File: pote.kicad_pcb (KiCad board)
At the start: 2 copper layers, 39.4 x 36.8 mm, 16 parts, among them J1 Conn_01x01, J2 Conn_01x01, J3 Conn_01x01, J4 Conn_01x01, J5 Conn_01x01, J6 Conn_01x01, J7 Conn_01x01, J8 Conn_01x01, U1 Opamp_Quad_Generic

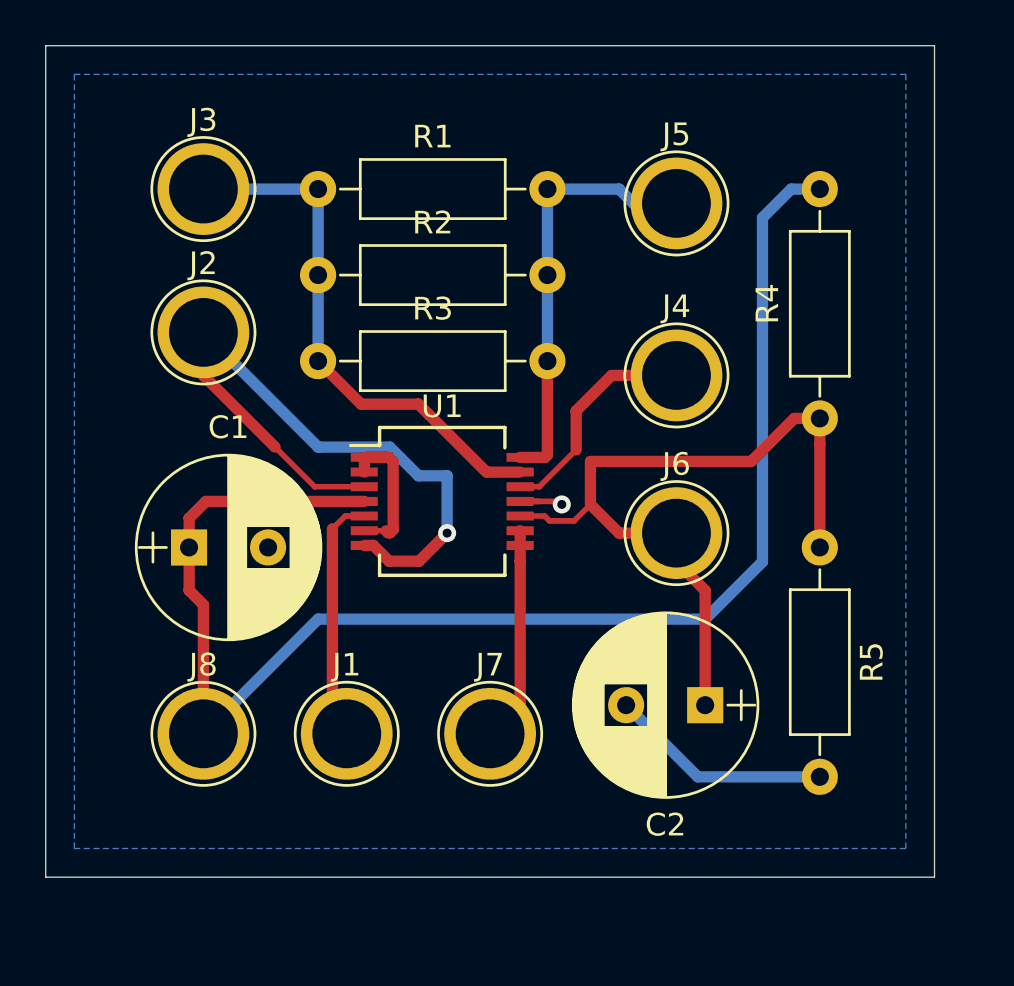
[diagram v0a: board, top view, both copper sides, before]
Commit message: Modified by kou
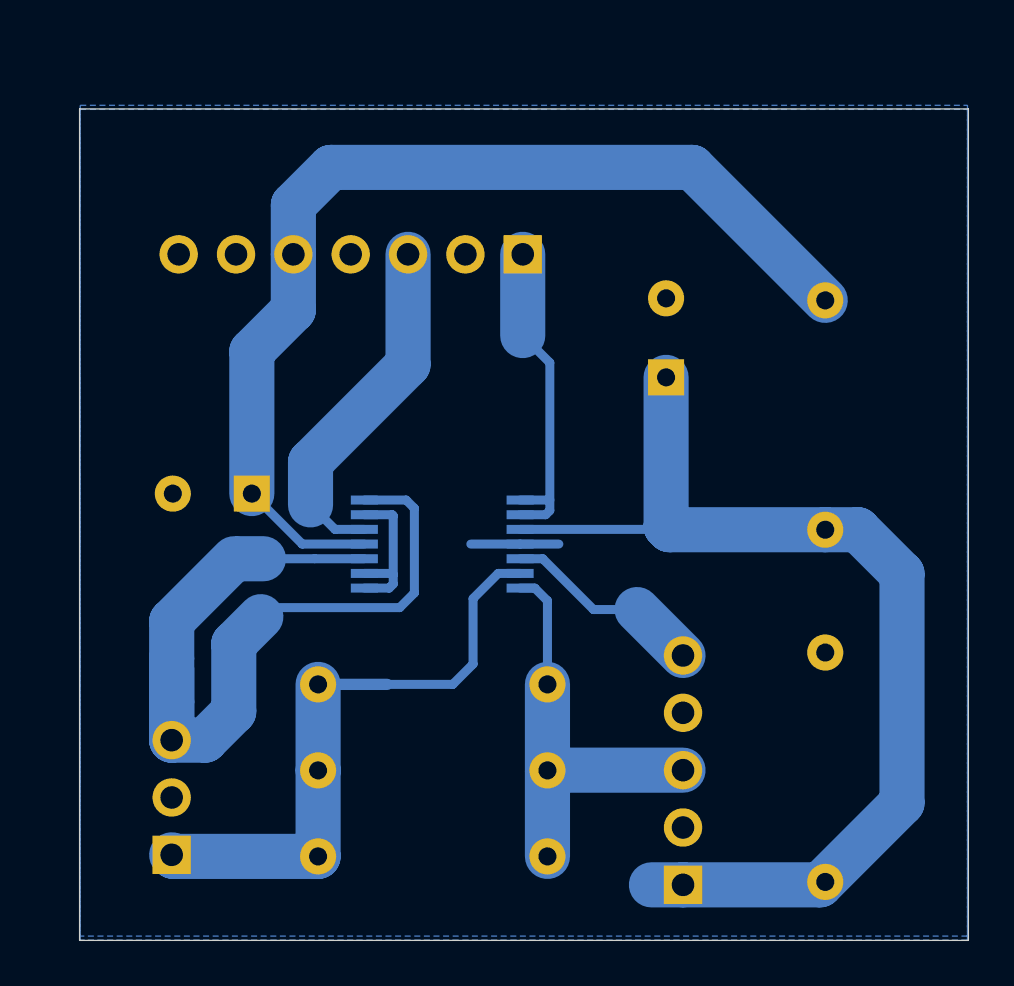
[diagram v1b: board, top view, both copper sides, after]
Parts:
- removed J4, J5, J6, J7, J8: Conn_01x01, Connectors:1pin
- C1, C2, R1, R2, R3, R4, R5, U1: moved to B.Cu
- J1: value Conn_01x01 -> Conn_01x03; footprint Connectors:1pin -> Connector_PinHeader_2.54mm:PinHeader_1x03_P2.54mm_Vertical; moved to B.Cu
- J2: value Conn_01x01 -> Conn_01x03; footprint Connectors:1pin -> Connector_PinHeader_2.54mm:PinHeader_1x07_P2.54mm_Vertical; moved to B.Cu
- J3: value Conn_01x01 -> Conn_01x03; footprint Connectors:1pin -> Connector_PinHeader_2.54mm:PinHeader_1x05_P2.54mm_Vertical; moved to B.Cu
- moved J3 37.4 mm to (181.9, 105.8)
- moved R1 29.6 mm to (165.7, 104.5)
- moved R2 21.9 mm to (165.7, 100.7)
- moved R5 14.8 mm to (188.2, 105.6), turned to 90 degrees
- moved C2 14.6 mm to (181.2, 83.3), turned to 90 degrees
- moved J2 14.6 mm to (174.8, 77.8), turned to 90 degrees
- moved R3 14.3 mm to (165.7, 96.9)
- moved J1 9.43 mm to (159.2, 104.4)
- moved R4 4.94 mm to (188.2, 90.0)
- moved C1 3.66 mm to (162.8, 88.4), turned to 180 degrees
- moved U1 1.89 mm to (171.2, 90.7)
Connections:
- J3 pad 1: Net-(J3-Pad1) -> Net-(C2-Pad1)
- R1 pad 1: Net-(J3-Pad1) -> Net-(J1-Pad1)
- R1 pad 2: Net-(J5-Pad1) -> Net-(J3-Pad3)
- R2 pad 1: Net-(J3-Pad1) -> Net-(J1-Pad1)
- R2 pad 2: Net-(J5-Pad1) -> Net-(J3-Pad3)
- R3 pad 1: Net-(J3-Pad1) -> Net-(J1-Pad1)
- R3 pad 2: Net-(J5-Pad1) -> Net-(J3-Pad3)
- U1 pad 12: Net-(J4-Pad1) -> Net-(J3-Pad5)
- U1 pad 13: Net-(J3-Pad1) -> Net-(J1-Pad1)
- U1 pad 14: Net-(J5-Pad1) -> Net-(J3-Pad3)
- U1 pad 3: Net-(J2-Pad1) -> Net-(J1-Pad3)
- U1 pad 5: Net-(J1-Pad1) -> Net-(J2-Pad3)
- U1 pad 7: Net-(J2-Pad1) -> Net-(J1-Pad3)
- U1 pad 8: Net-(J7-Pad1) -> Net-(J2-Pad1)
- U1 pad 9: Net-(J7-Pad1) -> Net-(J2-Pad1)
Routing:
- net Net-(J1-Pad3): track 0.00 -> 40.9 mm
- net Net-(J3-Pad1): track 23.7 -> 0.00 mm
- net Net-(J5-Pad1): track 19.0 -> 0.00 mm
- net Net-(J3-Pad3): track 0.00 -> 18.8 mm
- net VCC: track 64.1 -> 46.1 mm
- net Net-(J2-Pad1): track 31.5 -> 14.6 mm, vias 1 -> 0
- net Net-(J1-Pad1): track 11.0 -> 26.8 mm
- net Net-(J2-Pad3): track 0.00 -> 15.7 mm
- net Net-(C2-Pad1): track 34.6 -> 47.5 mm
- net Net-(J4-Pad1): track 9.98 -> 0.00 mm
- net Net-(J7-Pad1): track 9.55 -> 0.00 mm
- net Net-(J3-Pad5): track 0.00 -> 8.99 mm
- net GNDA: track 12.6 -> 3.90 mm, vias 1 -> 0
